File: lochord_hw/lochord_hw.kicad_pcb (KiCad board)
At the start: 2 copper layers, 29 x 51.9 mm, 21 parts, among them J1 TYPE-C-31-M-12, J2 Conn_01x20_Pin, J3 Conn_01x20_Pin, SW1 TS-1088-AR02016, SW2 TS-1088-AR02016, U2 ESP32-S3-WROOM-1, U3 LD1117S33TR_SOT223

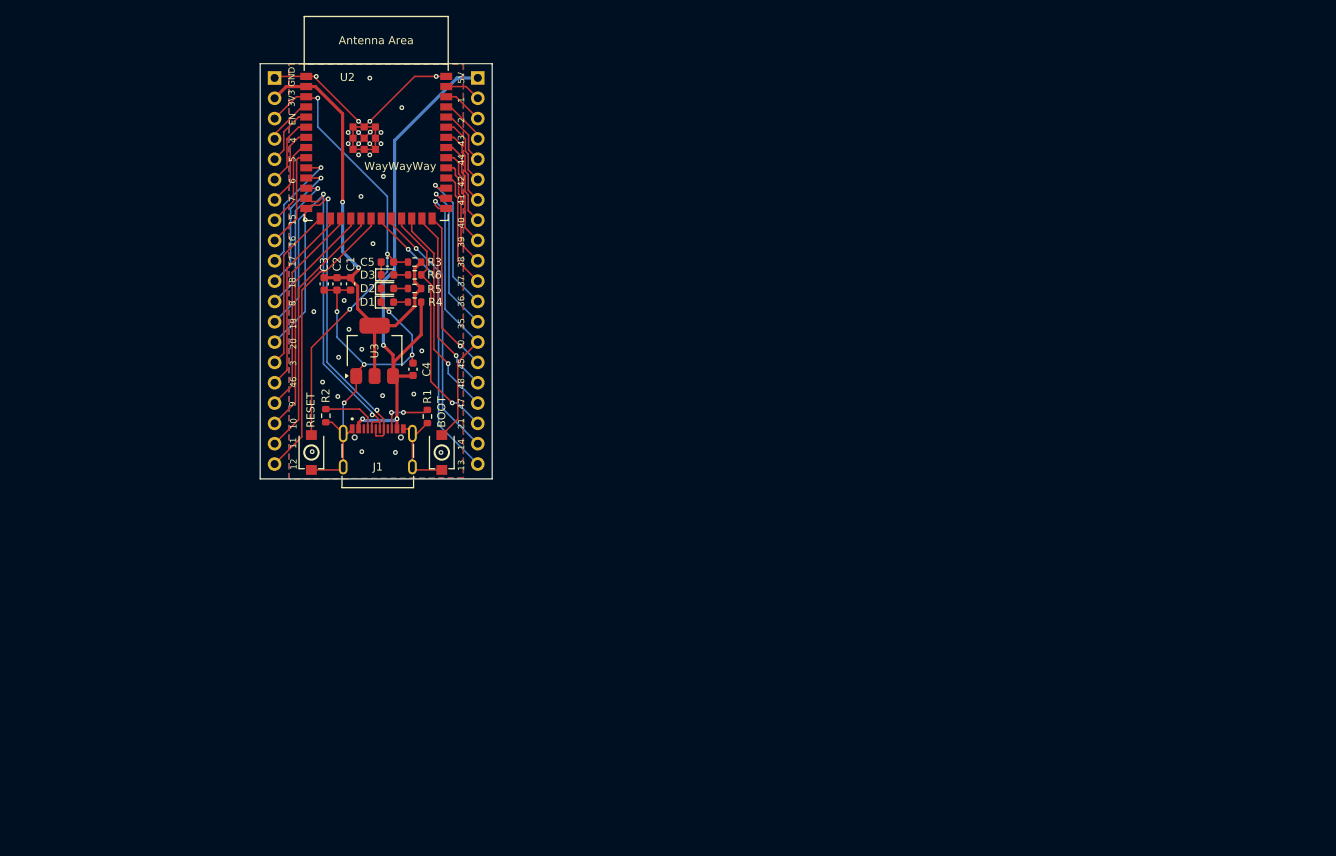
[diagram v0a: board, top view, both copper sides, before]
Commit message: atomic14 pcb design
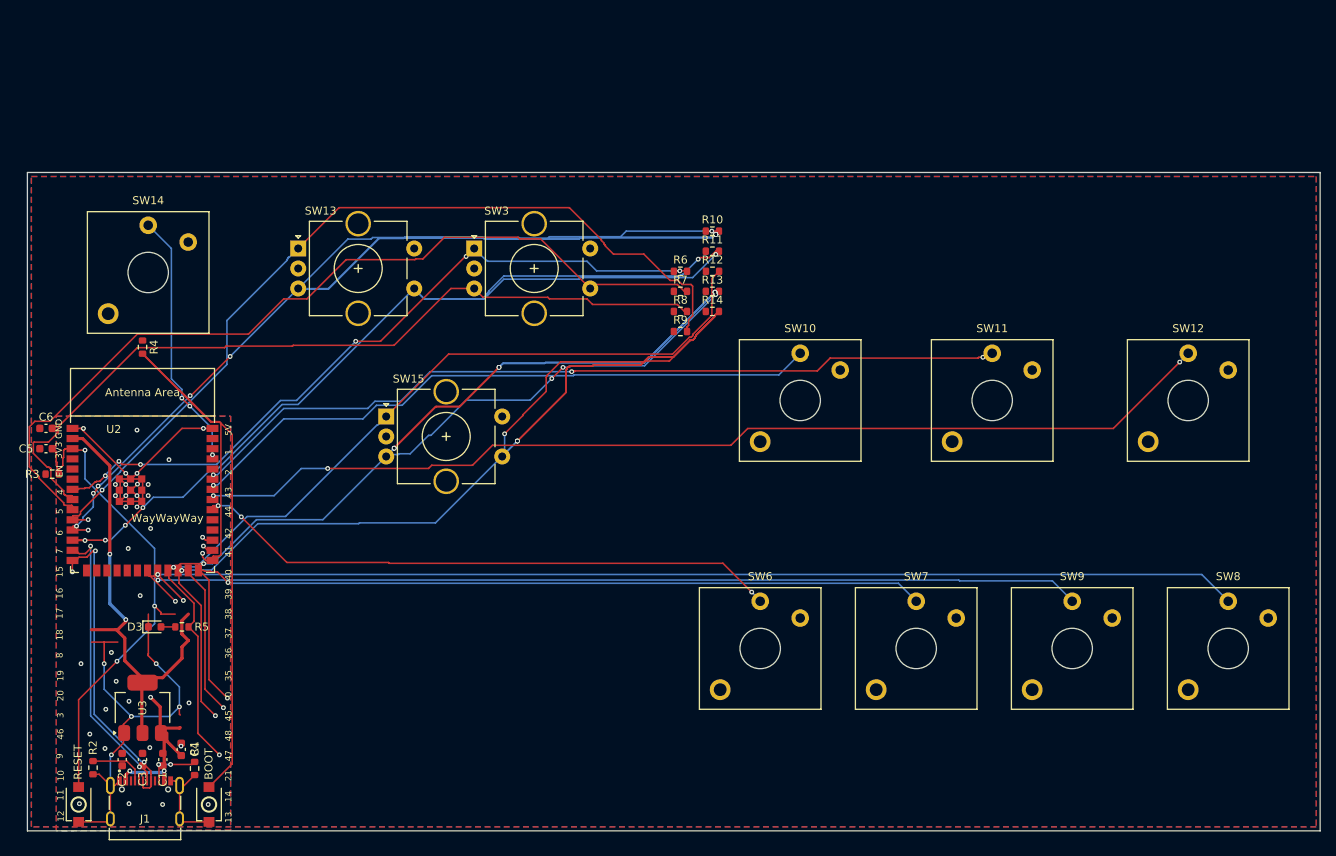
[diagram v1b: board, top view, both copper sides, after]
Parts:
- removed D1: RED, LED_SMD:LED_0603_1608Metric
- removed D2: GREEN, LED_SMD:LED_0603_1608Metric
- removed J2, J3: Conn_01x20_Pin, Connector_PinHeader_2.54mm:PinHeader_1x20_P2.54mm_Vertical
- removed the R5 at (131.8, 69.5)
- added C6: 100nF, Capacitor_SMD:C_0603_1608Metric, F.Cu at (85.7, 87.0)
- added R10: 10K, Resistor_SMD:R_0603_1608Metric, F.Cu at (169.0, 62.3)
- added R11: 10K, Resistor_SMD:R_0603_1608Metric, F.Cu at (169.0, 64.8)
- added R12: 10K, Resistor_SMD:R_0603_1608Metric, F.Cu at (169.0, 67.3)
- added R13: 10K, Resistor_SMD:R_0603_1608Metric, F.Cu at (169.0, 69.9)
- added R14: 10K, Resistor_SMD:R_0603_1608Metric, F.Cu at (169.0, 72.4)
- added R6: 10K, Resistor_SMD:R_0603_1608Metric, F.Cu at (165.0, 67.3)
- added R7: 10K, Resistor_SMD:R_0603_1608Metric, F.Cu at (165.0, 69.9)
- added R8: 10K, Resistor_SMD:R_0603_1608Metric, F.Cu at (165.0, 72.4)
- added R9: 10K, Resistor_SMD:R_0603_1608Metric, F.Cu at (165.0, 74.9)
- added SW10: SW_Push, Switch_Keyboard_Kailh:SW_Kailh_Choc_V2_1.50u, F.Cu at (180.0, 83.5)
- added SW11: SW_Push, Switch_Keyboard_Kailh:SW_Kailh_Choc_V2_1.00u, F.Cu at (204.0, 83.5)
- added SW12: SW_Push, Switch_Keyboard_Kailh:SW_Kailh_Choc_V2_1.50u, F.Cu at (228.5, 83.5)
- added SW13: UI_Encoder, Rotary_Encoder:RotaryEncoder_Alps_EC11E-Switch_Vertical_H20mm_CircularMountingHoles, F.Cu at (117.2, 64.5)
- added SW14: SW_Push, Switch_Keyboard_Kailh:SW_Kailh_Choc_V2_1.00u, F.Cu at (98.5, 67.5)
- added SW15: UI_Encoder, Rotary_Encoder:RotaryEncoder_Alps_EC11E-Switch_Vertical_H20mm_CircularMountingHoles, F.Cu at (128.2, 85.5)
- added SW3: UI_Encoder, Rotary_Encoder:RotaryEncoder_Alps_EC11E-Switch_Vertical_H20mm_CircularMountingHoles, F.Cu at (139.2, 64.5)
- added SW6: SW_Push, Switch_Keyboard_Kailh:SW_Kailh_Choc_V2_2.25u_90deg, F.Cu at (175.0, 114.5)
- added SW7: SW_Push, Switch_Keyboard_Kailh:SW_Kailh_Choc_V2_2.25u_90deg, F.Cu at (194.5, 114.5)
- added SW8: SW_Push, Switch_Keyboard_Kailh:SW_Kailh_Choc_V2_2.25u_90deg, F.Cu at (233.5, 114.5)
- added SW9: SW_Push, Switch_Keyboard_Kailh:SW_Kailh_Choc_V2_2.25u_90deg, F.Cu at (214.0, 114.5)
- C1: value 10u -> 10uF
- C2: value 22u -> 22uF
- C3: value 100n -> 100nF
- C4: value 10u -> 100nF
- C5: value 10u -> 1uF
- D3: value BLUE -> RED
- R3, R4: value 5.1K -> 10K
- R5: renamed from R6; value 5.1K -> 1K
- U2: value ESP32-S3-WROOM-1 -> ESP32-S3-WROOM-1-N8R8
- moved C2 65.2 mm to (95.2, 128.4), turned to 90 degrees
- moved C1 63.9 mm to (100.3, 128.4), turned to 90 degrees
- moved C3 63.6 mm to (97.8, 128.4), turned to 90 degrees
- moved C4 55.7 mm to (102.6, 127.1)
- moved U3 53.2 mm to (97.8, 121.9)
- moved U2 52.8 mm to (97.8, 95.2)
- moved J1 52.8 mm to (98.1, 135.8)
- moved R1 52.8 mm to (104.3, 129.5)
- moved R2 52.8 mm to (91.6, 129.4)
- moved SW1 52.8 mm to (89.8, 134.0)
- moved D3 52.8 mm to (99.3, 111.8)
- moved R5 52.8 mm to (102.7, 111.8)
- moved SW2 52.8 mm to (106.1, 134.0)
- moved R3 52.5 mm to (86.5, 92.7), turned to 0 degrees
- moved C5 48.6 mm to (85.7, 89.5)
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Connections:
- R4 pad 1: +5V -> +3V3
- R4 pad 2: Net-(D1-A) -> GPIO0
- R5 pad 1: GPIO21 -> +3V3
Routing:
- net GPIO18: track 17.1 -> 322.7 mm, vias 1 -> 11
- net GPIO47: track 26.5 -> 202.7 mm, vias 1 -> 11
- net GPIO48: track 23.4 -> 176.0 mm, vias 1 -> 5
- net GPIO8: track 17.8 -> 139.6 mm, vias 1 -> 6
- net GPIO40: track 11.2 -> 129.8 mm, vias 0 -> 3
- net GPIO14: track 32.6 -> 140.7 mm, vias 1 -> 2
- net GPIO16: track 12.5 -> 108.4 mm
- net GPIO42: track 8.73 -> 104.3 mm, vias 0 -> 3
- net GPIO17: track 15.9 -> 109.6 mm, vias 1 -> 2
- net GPIO15: track 11.0 -> 101.1 mm
- net GPIO45: track 20.5 -> 108.7 mm, vias 1 -> 2
- net GPIO13: track 35.7 -> 122.7 mm, vias 1 -> 2
- net GPIO21: track 30.5 -> 113.5 mm, vias 1 -> 2
- net GPIO7: track 10.0 -> 90.8 mm, vias 0 -> 6
- net GPIO41: track 10.0 -> 80.8 mm, vias 0 -> 1
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- added copper zone on F.Cu, net +3V3
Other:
- board size 29 x 51.9 mm -> 161.6 x 82.3 mm
